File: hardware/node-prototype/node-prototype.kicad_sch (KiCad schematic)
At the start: 0 parts

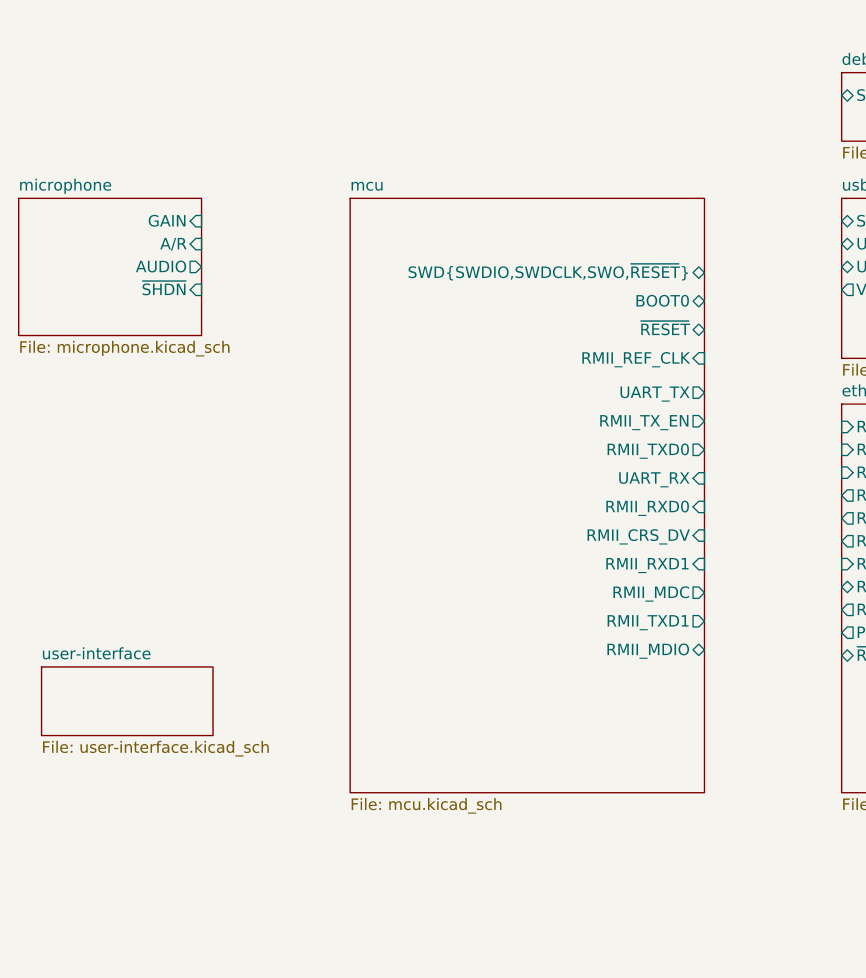
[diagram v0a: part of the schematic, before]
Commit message: WIP on user interface
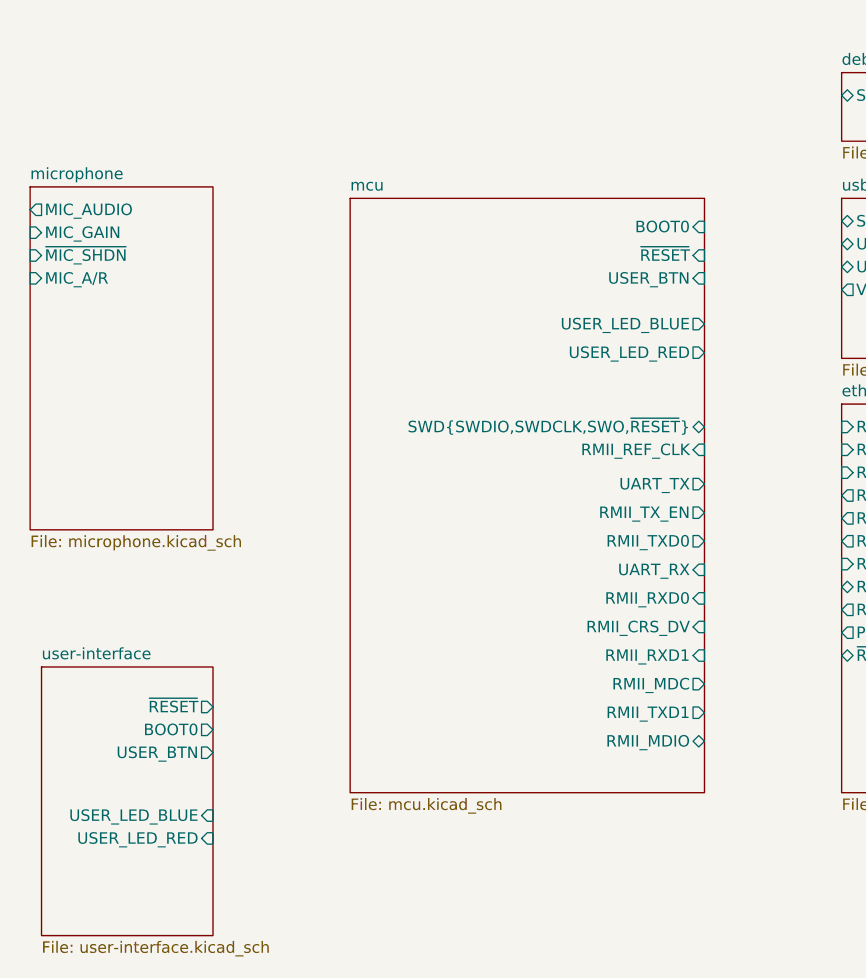
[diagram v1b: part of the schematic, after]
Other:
- sheet mcu ports: added USER_BTN, USER_LED_BLUE, USER_LED_RED; removed none
- sheet microphone ports: added MIC_AUDIO, MIC_A/R, MIC_GAIN, ~{MIC_SHDN}; removed AUDIO, A/R, GAIN, ~{SHDN}
- sheet user-interface ports: added BOOT0, USER_BTN, USER_LED_BLUE, USER_LED_RED, ~{RESET}; removed none
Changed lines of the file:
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@@
     (effects (font (size 1.27 1.27)) (justify left bottom))
   )
-  (sheet (at 63.5 100.33) (size 19.05 7.62) (fields_autoplaced)
+  (sheet (at 63.5 100.33) (size 19.05 29.845) (fields_autoplaced)
     (stroke (width 0.1524) (type solid))
     (fill (color 0 0 0 0.0000))
@@
       (effects (font (size 1.27 1.27)) (justify left bottom))
     )
-    (property "Sheetfile" "user-interface.kicad_sch" (at 63.5 108.5346 0)
-      (effects (font (size 1.27 1.27)) (justify left top))
+    (property "Sheetfile" "user-interface.kicad_sch" (at 63.5 130.7596 0)
+      (effects (font (size 1.27 1.27)) (justify left top))
+    )
+    (pin "BOOT0" output (at 82.55 107.315 0)
+      (effects (font (size 1.27 1.27)) (justify right))
+    )
+    (pin "USER_LED_RED" input (at 82.55 119.38 0)
+      (effects (font (size 1.27 1.27)) (justify right))
+    )
+    (pin "USER_BTN" output (at 82.55 109.855 0)
+      (effects (font (size 1.27 1.27)) (justify right))
+    )
+    (pin "USER_LED_BLUE" input (at 82.55 116.84 0)
+      (effects (font (size 1.27 1.27)) (justify right))
+    )
+    (pin "~{RESET}" output (at 82.55 104.775 0)
+      (effects (font (size 1.27 1.27)) (justify right))
     )
     (instances
@@
     )
   )
-  (sheet (at 60.96 48.26) (size 20.32 15.24) (fields_autoplaced)
-    (stroke (width 0.1524) (type solid))
-    (fill (color 0 0 0 0.0000))
-    (property "Sheetname" "microphone" (at 60.96 47.5484 0)
-      (effects (font (size 1.27 1.27)) (justify left bottom))
-    )
-    (property "Sheetfile" "microphone.kicad_sch" (at 60.96 64.0846 0)
-      (effects (font (size 1.27 1.27)) (justify left top))
-    )
-    (pin "GAIN" input (at 81.28 50.8 0)
-      (effects (font (size 1.27 1.27)) (justify right))
-    )
-    (pin "A{slash}R" input (at 81.28 53.34 0)
-      (effects (font (size 1.27 1.27)) (justify right))
-    )
-    (pin "AUDIO" output (at 81.28 55.88 0)
-      (effects (font (size 1.27 1.27)) (justify right))
-    )
-    (pin "~{SHDN}" input (at 81.28 58.42 0)
-      (effects (font (size 1.27 1.27)) (justify right))
+  (sheet (at 62.23 46.99) (size 20.32 38.1) (fields_autoplaced)
+    (stroke (width 0.1524) (type solid))
+    (fill (color 0 0 0 0.0000))
+    (property "Sheetname" "microphone" (at 62.23 46.2784 0)
+      (effects (font (size 1.27 1.27)) (justify left bottom))
+    )
+    (property "Sheetfile" "microphone.kicad_sch" (at 62.23 85.6746 0)
+      (effects (font (size 1.27 1.27)) (justify left top))
+    )
+    (pin "MIC_GAIN" input (at 62.23 52.07 180)
+      (effects (font (size 1.27 1.27)) (justify left))
+    )
+    (pin "MIC_AUDIO" output (at 62.23 49.53 180)
+      (effects (font (size 1.27 1.27)) (justify left))
+    )
+    (pin "~{MIC_SHDN}" input (at 62.23 54.61 180)
+      (effects (font (size 1.27 1.27)) (justify left))
+    )
+    (pin "MIC_A{slash}R" input (at 62.23 57.15 180)
+      (effects (font (size 1.27 1.27)) (justify left))
     )
     (instances
@@
       (effects (font (size 1.27 1.27)) (justify left top))
     )
-    (pin "SWD{SWDIO,SWDCLK,SWO,~{RESET}}" bidirectional (at 137.16 56.515 0)
-      (effects (font (size 1.27 1.27)) (justify right))
-    )
-    (pin "BOOT0" bidirectional (at 137.16 59.69 0)
-      (effects (font (size 1.27 1.27)) (justify right))
-    )
-    (pin "~{RESET}" bidirectional (at 137.16 62.865 0)
-      (effects (font (size 1.27 1.27)) (justify right))
-    )
-    (pin "RMII_REF_CLK" input (at 137.16 66.04 0)
-      (effects (font (size 1.27 1.27)) (justify right))
-    )
-    (pin "UART_TX" output (at 137.16 69.85 0)
-      (effects (font (size 1.27 1.27)) (justify right))
-    )
-    (pin "RMII_TX_EN" output (at 137.16 73.025 0)
-      (effects (font (size 1.27 1.27)) (justify right))
-    )
-    (pin "RMII_TXD0" output (at 137.16 76.2 0)
-      (effects (font (size 1.27 1.27)) (justify right))
-    )
-    (pin "UART_RX" input (at 137.16 79.375 0)
-      (effects (font (size 1.27 1.27)) (justify right))
-    )
-    (pin "RMII_RXD0" input (at 137.16 82.55 0)
-      (effects (font (size 1.27 1.27)) (justify right))
-    )
-    (pin "RMII_CRS_DV" input (at 137.16 85.725 0)
-      (effects (font (size 1.27 1.27)) (justify right))
-    )
-    (pin "RMII_RXD1" input (at 137.16 88.9 0)
-      (effects (font (size 1.27 1.27)) (justify right))
-    )
-    (pin "RMII_MDC" output (at 137.16 92.075 0)
-      (effects (font (size 1.27 1.27)) (justify right))
-    )
-    (pin "RMII_TXD1" output (at 137.16 95.25 0)
-      (effects (font (size 1.27 1.27)) (justify right))
-    )
-    (pin "RMII_MDIO" bidirectional (at 137.16 98.425 0)
-      (effects (font (size 1.27 1.27)) (justify right))
-    )
+    (pin "SWD{SWDIO,SWDCLK,SWO,~{RESET}}" bidirectional (at 137.16 73.66 0)
+      (effects (font (size 1.27 1.27)) (justify right))
+    )
+    (pin "BOOT0" input (at 137.16 51.435 0)
+      (effects (font (size 1.27 1.27)) (justify right))
+    )
+    (pin "~{RESET}" input (at 137.16 54.61 0)
+      (effects (font (size 1.27 1.27)) (justify right))
+    )
+    (pin "RMII_REF_CLK" input (at 137.16 76.2 0)
+      (effects (font (size 1.27 1.27)) (justify right))
+    )
+    (pin "UART_TX" output (at 137.16 80.01 0)
+      (effects (font (size 1.27 1.27)) (justify right))
+    )
+    (pin "RMII_TX_EN" output (at 137.16 83.185 0)
+      (effects (font (size 1.27 1.27)) (justify right))
+    )
+    (pin "RMII_TXD0" output (at 137.16 86.36 0)
+      (effects (font (size 1.27 1.27)) (justify right))
+    )
+    (pin "UART_RX" input (at 137.16 89.535 0)
+      (effects (font (size 1.27 1.27)) (justify right))
+    )
+    (pin "RMII_RXD0" input (at 137.16 92.71 0)
+      (effects (font (size 1.27 1.27)) (justify right))
+    )
+    (pin "RMII_CRS_DV" input (at 137.16 95.885 0)
+      (effects (font (size 1.27 1.27)) (justify right))
+    )
+    (pin "RMII_RXD1" input (at 137.16 99.06 0)
+      (effects (font (size 1.27 1.27)) (justify right))
+    )
+    (pin "RMII_MDC" output (at 137.16 102.235 0)
+      (effects (font (size 1.27 1.27)) (justify right))
+    )
+    (pin "RMII_TXD1" output (at 137.16 105.41 0)
+      (effects (font (size 1.27 1.27)) (justify right))
+    )
+    (pin "RMII_MDIO" bidirectional (at 137.16 108.585 0)
+      (effects (font (size 1.27 1.27)) (justify right))
+    )
+    (pin "USER_BTN" input (at 137.16 57.15 0)
+      (effects (font (size 1.27 1.27)) (justify right))
+    )
+    (pin "USER_LED_BLUE" output (at 137.16 62.23 0)
+      (effects (font (size 1.27 1.27)) (justify right))
+    )
+    (pin "USER_LED_RED" output (at 137.16 65.405 0)
+      (effects (font (size 1.27 1.27)) (justify right))
+    )
